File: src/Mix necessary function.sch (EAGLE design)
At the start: 26 parts, among them SW1 02-JST, SW2 02-JST

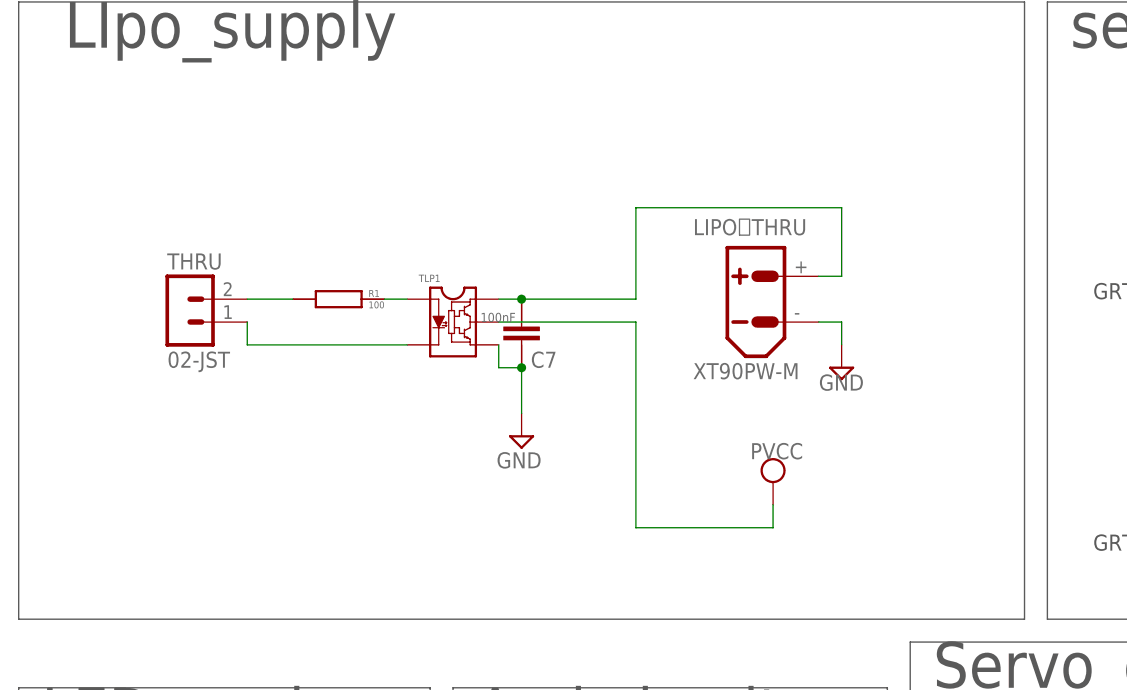
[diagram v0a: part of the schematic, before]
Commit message: fix
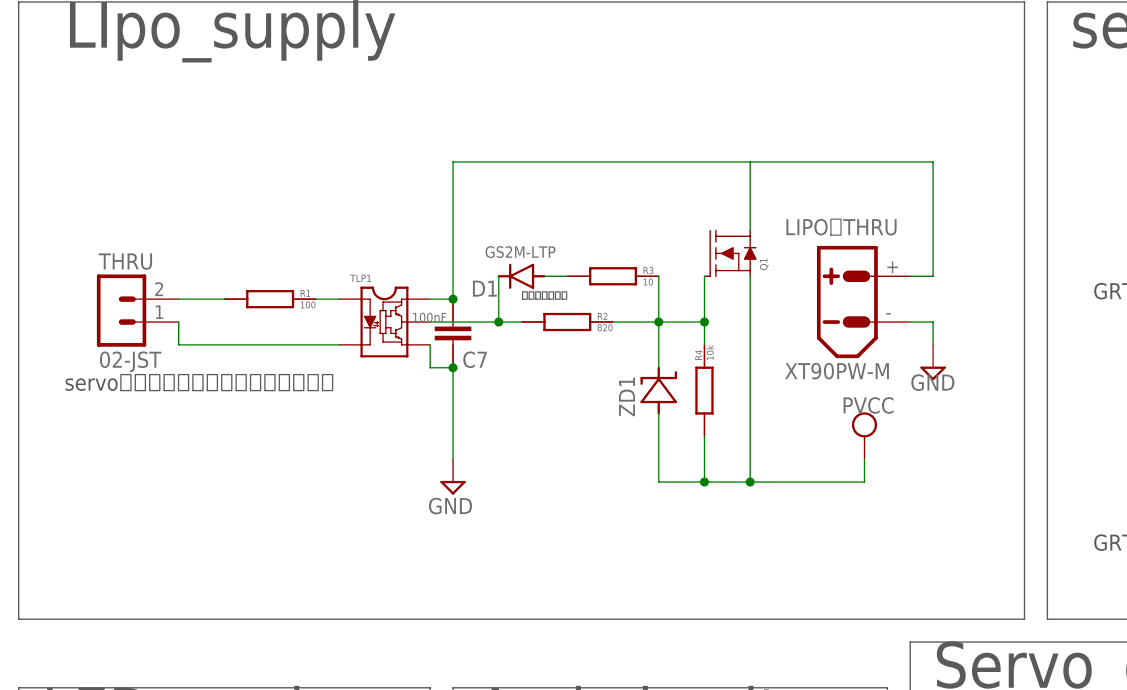
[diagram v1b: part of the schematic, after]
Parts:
- added D1: GS2M-LTP, GS2M-LTP:GS2M-LTP
- added Q1: SQJA16EP-T1_GE3, SQJA16EP-T1_GE3:SQJA16EP-T1_GE3
- added R2: 820, CR0603:CR0603
- added R3: 10, CR0603:CR0603
- added R4: 10k, CR0603:CR0603
- added ZD1: MMBZ5248B-TP, MMBZ5248B-TP:MMBZ5248B-TP
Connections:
- new net N$6: D1.C, R2.LEFT, TLP1.VOUT
- new net N$7: Q1.G, R2.RIGHT, R3.RIGHT, R4.RIGHT, ZD1.C
- new net N$8: D1.A, R3.LEFT
- net N$20: now also Q1.D
- net PVCC: now also Q1.S, R4.LEFT, ZD1.A; no longer TLP1.VOUT
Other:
- note added: "servoの非常停止機能の接続用コネクタ"
- note added: "逆方向漏れ防止"
- moved on the sheet: C7, LIPO＿THRU, R1, THRU, TLP1
